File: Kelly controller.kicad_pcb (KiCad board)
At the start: 2 copper layers, 104.5 x 91 mm, 48 parts, among them J1 Conn_01x06_Female, J11 Conn_01x06_Female, J12 Conn_01x06_Female, J2 Conn_01x06_Female, J3 I2C throttle, J4 throttle A, J5 throttle B, J6 Board power, J7 B_5_12_48, J8 A_5_12_48, SW1 FNR, SW2 Brake_SW, SW4 Power Switch, SW5 Power Switch, U1 LTV-247, U2 LTV-247, U3 MCP4251, U4 SPAN02C-05

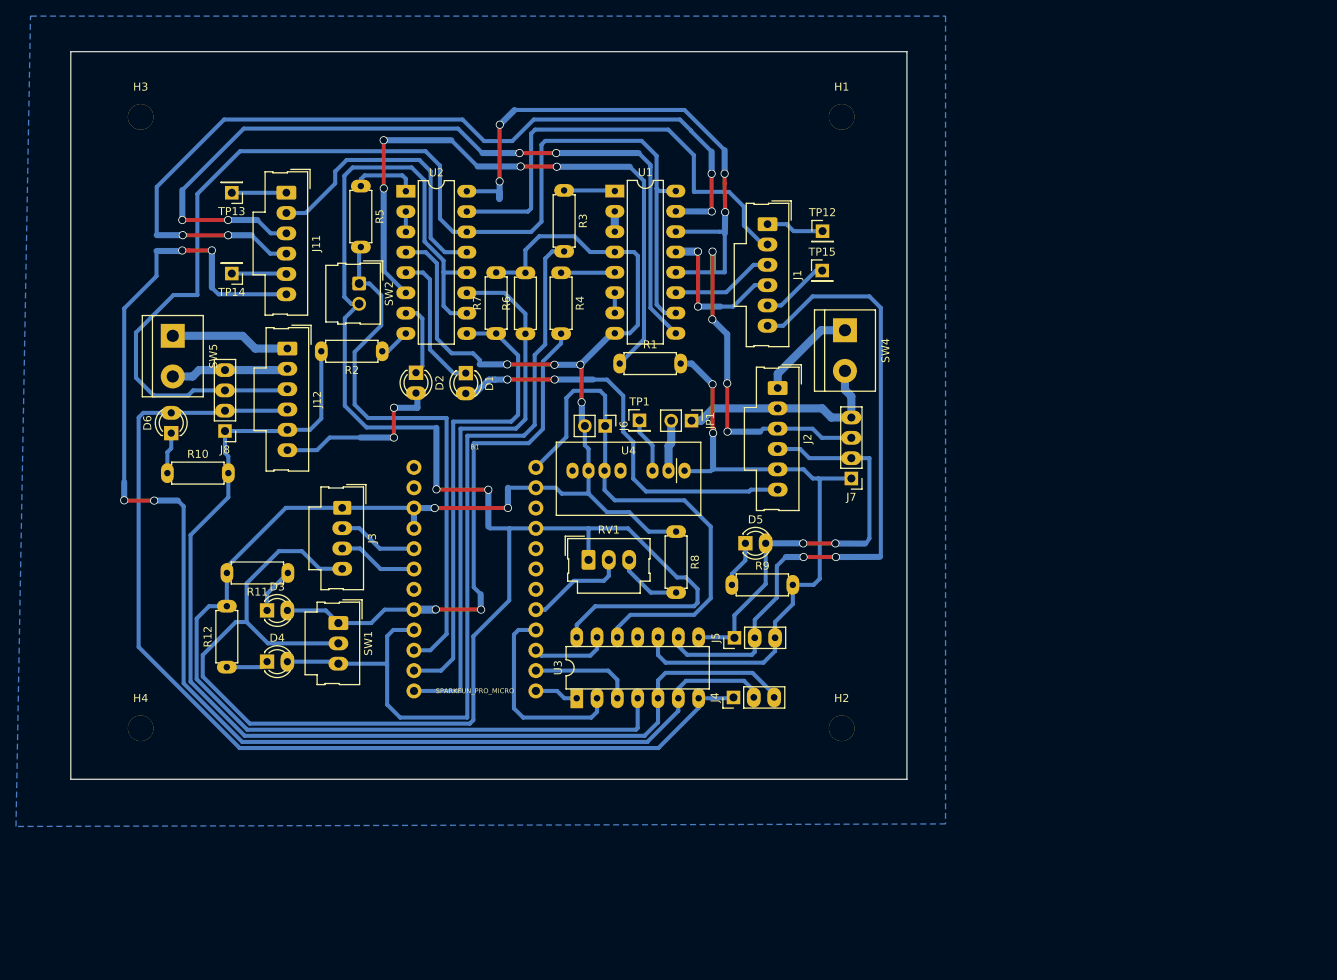
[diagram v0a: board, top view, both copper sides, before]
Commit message: board ready to cut
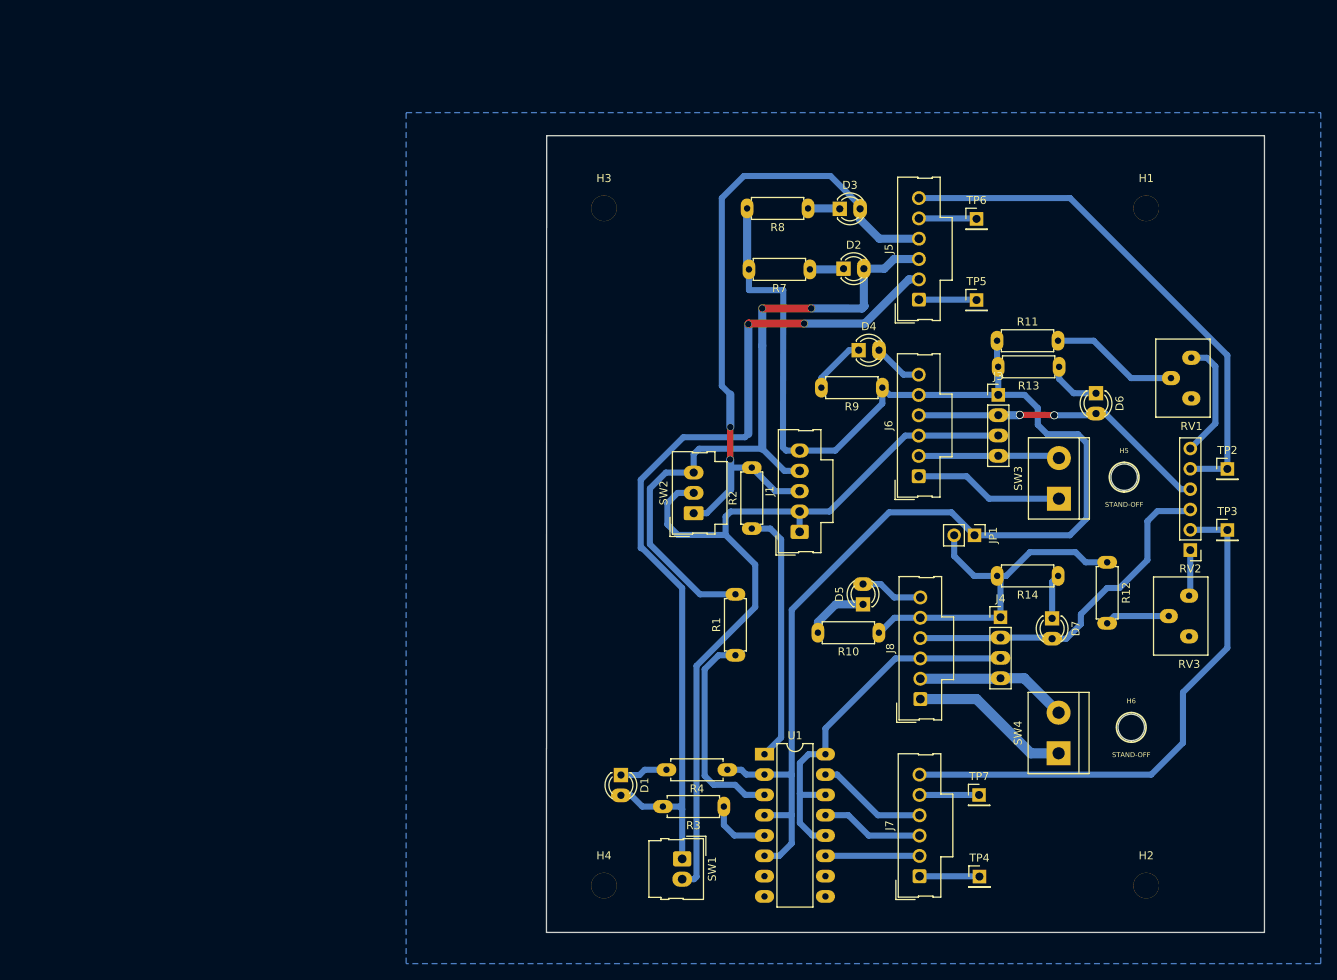
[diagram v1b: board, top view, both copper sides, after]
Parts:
- removed B1: SPARKFUN_PRO_MICRO, Boards:SPARKFUN_PRO_MICRO
- removed J11, J12, J2: Conn_01x06_Female, myfootprints:Molex_SL_171971-0006_1x06_P2.54mm_Vertical
- removed R5: 220, myfootprints:R_Axial_DIN0207_L6.3mm_D2.5mm_P7.62mm_Horizontal_wide_pads
- removed R6: 10k, myfootprints:R_Axial_DIN0207_L6.3mm_D2.5mm_P7.62mm_Horizontal_wide_pads
- removed SW5: Power Switch, TerminalBlock:TerminalBlock_bornier-2_P5.08mm
- removed TP1: RC, Connector_PinHeader_2.54mm:PinHeader_1x01_P2.54mm_Vertical
- removed TP12, TP13: ftsw, Connector_PinHeader_2.54mm:PinHeader_1x01_P2.54mm_Vertical
- removed TP14, TP15: anbrk, Connector_PinHeader_2.54mm:PinHeader_1x01_P2.54mm_Vertical
- removed U2: LTV-247, Package_DIP:DIP-16_W7.62mm_LongPads
- removed U3: MCP4251, Package_DIP:DIP-14_W7.62mm
- removed U4: SPAN02C-05, myfootprints:SPAN02
- added D7: RED, myfootprints:LED_D3.0mm_wide_pads, F.Cu at (215.5, 117.3)
- added H5: STAND-OFF, Hardware:STAND-OFF, F.Cu at (224.5, 99.6)
- added H6: STAND-OFF, Hardware:STAND-OFF, F.Cu at (225.4, 130.9)
- added R13: 1k, myfootprints:R_Axial_DIN0207_L6.3mm_D2.5mm_P7.62mm_Horizontal_wide_pads, F.Cu at (216.4, 85.9)
- added R14: 1k, myfootprints:R_Axial_DIN0207_L6.3mm_D2.5mm_P7.62mm_Horizontal_wide_pads, F.Cu at (216.3, 112.0)
- added RV2: throttle(10k), Connector_PinHeader_2.54mm:PinHeader_1x06_P2.54mm_Vertical, F.Cu at (232.8, 108.8)
- added RV3: trim(1k), myfootprints:trimpot_breadboard_spacing, F.Cu at (232.7, 114.5)
- added SW3: Power Switch, TerminalBlock:TerminalBlock_bornier-2_P5.08mm, F.Cu at (216.4, 102.3)
- added TP2: T_A, Connector_PinHeader_2.54mm:PinHeader_1x01_P2.54mm_Vertical, F.Cu at (237.4, 98.6)
- added TP3: T_B, Connector_PinHeader_2.54mm:PinHeader_1x01_P2.54mm_Vertical, F.Cu at (237.4, 106.2)
- added TP4: ftsw, Connector_PinHeader_2.54mm:PinHeader_1x01_P2.54mm_Vertical, F.Cu at (206.5, 149.6)
- added TP5: ftsw, Connector_PinHeader_2.54mm:PinHeader_1x01_P2.54mm_Vertical, F.Cu at (206.1, 77.5)
- added TP6: anbrk, Connector_PinHeader_2.54mm:PinHeader_1x01_P2.54mm_Vertical, F.Cu at (206.1, 67.4)
- added TP7: anbrk, Connector_PinHeader_2.54mm:PinHeader_1x01_P2.54mm_Vertical, F.Cu at (206.4, 139.4)
- D2: value yellow -> green
- D4: value green -> yellow
- D5: value RED -> yellow
- J1: value Conn_01x06_Female -> FNR switch; footprint myfootprints:Molex_SL_171971-0006_1x06_P2.54mm_Vertical -> Connector_Molex:Molex_SL_171971-0005_1x05_P2.54mm_Vertical
- J3: value I2C throttle -> A_5_12_48; footprint myfootprints:Molex_SL_171971-0004_1x04_P2.54mm_Vertical_wide_pads -> myfootprints:PinHeader_1x04_P2.54mm_Vertical_wide_pads
- J4: value throttle A -> B_5_12_48; footprint myfootprints:PinHeader_1x03_P2.54mm_Vertical_wide_pads -> myfootprints:PinHeader_1x04_P2.54mm_Vertical_wide_pads
- J5: value throttle B -> Conn_01x06_Female; footprint myfootprints:PinHeader_1x03_P2.54mm_Vertical_wide_pads -> Connector_Molex:Molex_SL_171971-0006_1x06_P2.54mm_Vertical
- J6: value Board power -> Conn_01x06_Female; footprint Connector_PinHeader_2.54mm:PinHeader_1x02_P2.54mm_Vertical -> Connector_Molex:Molex_SL_171971-0006_1x06_P2.54mm_Vertical
- J7: value B_5_12_48 -> Conn_01x06_Female; footprint myfootprints:PinHeader_1x04_P2.54mm_Vertical_wide_pads -> Connector_Molex:Molex_SL_171971-0006_1x06_P2.54mm_Vertical
- J8: value A_5_12_48 -> Conn_01x06_Female; footprint myfootprints:PinHeader_1x04_P2.54mm_Vertical_wide_pads -> Connector_Molex:Molex_SL_171971-0006_1x06_P2.54mm_Vertical
- JP1: value Jumper -> Jumper_2_Open
- R3: value 220 -> 1k
- R4: value 220 -> 2.2k
- R7: value 10k -> 2.2k
- R8: value 1k -> 2.2k
- RV1: value Throttle -> trim(1k); footprint myfootprints:Molex_SL_171971-0003_1x03_P2.54mm_Vertical_wide_pads -> myfootprints:trimpot_breadboard_spacing
- SW1: value FNR -> Brake_SW; footprint myfootprints:Molex_SL_171971-0003_1x03_P2.54mm_Vertical_wide_pads -> Connector_Molex:Molex_SL_171971-0002_1x02_P2.54mm_Vertical
- SW2: value Brake_SW -> FNR; footprint Connector_Molex:Molex_SL_171971-0002_1x02_P2.54mm_Vertical -> myfootprints:Molex_SL_171971-0003_1x03_P2.54mm_Vertical_wide_pads
- moved D6 115.7 mm to (221.0, 89.2), turned to 270 degrees
- moved R12 110.8 mm to (222.4, 110.3), turned to 270 degrees
- moved R11 93.3 mm to (208.6, 82.6), turned to 0 degrees
- moved J8 93.2 mm to (199.1, 127.4), turned to 90 degrees
- moved R10 91.1 mm to (193.9, 119.1), turned to 180 degrees
- moved D3 87.4 mm to (189.0, 66.1)
- moved D4 83.6 mm to (191.4, 83.8)
- moved J3 83.2 mm to (208.8, 89.4), turned to 0 degrees
- moved R3 79.6 mm to (174.5, 140.8), turned to 180 degrees
- moved RV1 79.5 mm to (232.9, 84.7), turned to 180 degrees
- moved U1 72.8 mm to (179.6, 134.3)
- moved R4 65.5 mm to (174.9, 136.2), turned to 180 degrees
- moved H4 61.2 mm to (159.5, 150.7)
- moved SW4 59.2 mm to (216.3, 134.2), turned to 90 degrees
- moved H3 59.0 mm to (159.5, 66.0)
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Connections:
- D1 pad 2: /Meter-B -> /Brake-A
- D2 pad 2: /Meter-A -> /REV-A
- D3 pad 2: /5-Reverse -> /FWD-A
- D4 pad 2: /6-Forward -> /Meter-A
- D5 pad 2: +5VB -> /Meter-B
- J1 pad 1: /Foot_SW-B -> +12VA
- J1 pad 2: /Brake-B -> +12VA
- J1 pad 3: /REV-B -> /FWD-A
- J1 pad 4: /FWD-B -> /REV-A
- J1 pad 5: /Brake_AN-B -> GNDA
- J3 pad 1: GND -> GNDA
- J3 pad 2: /SDA -> +5VA
- J3 pad 3: /SCL -> +12VA
- J3 pad 4: VCC -> +48VA
- J4 pad 1: +5VA -> GNDB
- J4 pad 2: /Throttle-A -> +5VB
- J4 pad 3: GNDA -> +12VB
- J5 pad 1: +5VB -> /Foot_SW-A
- J5 pad 2: /Throttle-B -> /Brake-A
- J5 pad 3: GNDB -> /REV-A
- J6 pad 1: 5V -> /PWR-A
- J6 pad 2: GND -> +48VA
- J7 pad 1: GNDB -> /Foot_SW-B
- J7 pad 2: +5VB -> /Brake-B
- J7 pad 3: +12VB -> /REV-B
- J7 pad 4: +48VB -> /FWD-B
- J8 pad 1: GNDA -> /PWR-B
- J8 pad 2: +5VA -> +48VB
- J8 pad 3: +12VA -> +12VB
- J8 pad 4: +48VA -> +5VB
- JP1 pad 1: +48VB -> GNDA
- JP1 pad 2: Net-(JP1-Pad2) -> GNDB
- R1 pad 2: GNDB -> /REV-A
- R10 pad 1: Net-(D6-Pad1) -> GNDB
- R10 pad 2: GNDA -> Net-(D5-Pad1)
- R11 pad 1: Net-(D3-Pad1) -> GNDA
- R11 pad 2: GND -> Net-(R11-Pad2)
- R12 pad 1: Net-(D4-Pad1) -> GNDB
- R12 pad 2: GND -> Net-(R12-Pad2)
- R2 pad 2: GNDA -> /FWD-A
- R3 pad 2: /6-Forward -> /Brake-A
- R4 pad 1: Net-(R4-Pad1) -> GNDA
- R4 pad 2: /5-Reverse -> Net-(D1-Pad1)
- R7 pad 1: /8-Meter_A -> Net-(D2-Pad1)
- R7 pad 2: GND -> GNDA
- R8 pad 1: GND -> Net-(D3-Pad1)
- R8 pad 2: Net-(R8-Pad2) -> GNDA
- R9 pad 1: Net-(D5-Pad1) -> GNDA
- R9 pad 2: GNDB -> Net-(D4-Pad1)
- RV1 pad 1: VCC -> Net-(RV1-Pad1)
- RV1 pad 2: Net-(B1-Pad17) -> Net-(R11-Pad2)
- RV1 pad 3: Net-(R8-Pad2) -> (no net)
- SW1 pad 1: /5-Reverse -> /Brake-A
- SW1 pad 2: VCC -> +12VA
- SW2 pad 1: /7-Brake -> /FWD-A
- SW2 pad 2: VCC -> +12VA
- U1 pad 1: Net-(R3-Pad1) -> Net-(R2-Pad1)
- U1 pad 10: +12VA -> (no net)
- U1 pad 11: /REV-B -> /Brake-B
- U1 pad 13: /FWD-B -> /REV-B
- U1 pad 15: /FWD-A -> /FWD-B
- U1 pad 16: +12VA -> +12VB
- U1 pad 2: Net-(U1-Pad2) -> GNDA
- U1 pad 3: Net-(U1-Pad2) -> Net-(R1-Pad1)
- U1 pad 4: GND -> GNDA
- U1 pad 5: Net-(R4-Pad1) -> Net-(R3-Pad1)
- U1 pad 6: Net-(U1-Pad6) -> GNDA
- U1 pad 7: Net-(U1-Pad6) -> (no net)
- U1 pad 8: GND -> (no net)
- U1 pad 9: /REV-A -> (no net)
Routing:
- net VCC: track 253.2 -> 0.00 mm, vias 2 -> 0
- net GND: track 235.2 -> 0.00 mm, vias 6 -> 0
- net /6-Forward: track 103.8 -> 0.00 mm
- net /Throttle-A: track 164.5 -> 65.5 mm, vias 4 -> 0
- net +5VA: track 130.6 -> 38.0 mm, vias 0 -> 2
- net /Brake-A: track 35.8 -> 111.2 mm, vias 0 -> 2
- net /5-Reverse: track 69.0 -> 0.00 mm, vias 2 -> 0
- net /9-Meter_B: track 68.8 -> 0.00 mm
- net +12VB: track 114.9 -> 47.0 mm, vias 8 -> 0
- net /7-Brake: track 67.9 -> 0.00 mm
- net 5V: track 66.0 -> 0.00 mm
- net /8-Meter_A: track 58.6 -> 0.00 mm
- net Net-(R1-Pad1): track 79.0 -> 26.4 mm, vias 4 -> 0
- net GNDA: track 138.1 -> 186.8 mm
- net /Brake-B: track 57.3 -> 11.8 mm
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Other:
- board size 104.5 x 91 mm -> 89.8 x 99.6 mm
